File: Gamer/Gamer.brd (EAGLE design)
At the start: 168.9 x 63.5 mm, 44 parts, among them J1 HEADER-1X8, J2 HEADER-1X8, J3 HEADER-1X8, J4 HEADER-1X8, J5 HEADER-1X8, J6 HEADER-1X8, J7 HEADER-1X8, J8 HEADER-1X8, U1 MMA8653FCR1, U2 ATTINY48, U3 ULN2803AFWG, U4 ATTINY48, U5 ULN2803AFWG, U6 ATTINY48, U7 ULN2803AFWG, U8 ATTINY48, U9 ULN2803AFWG

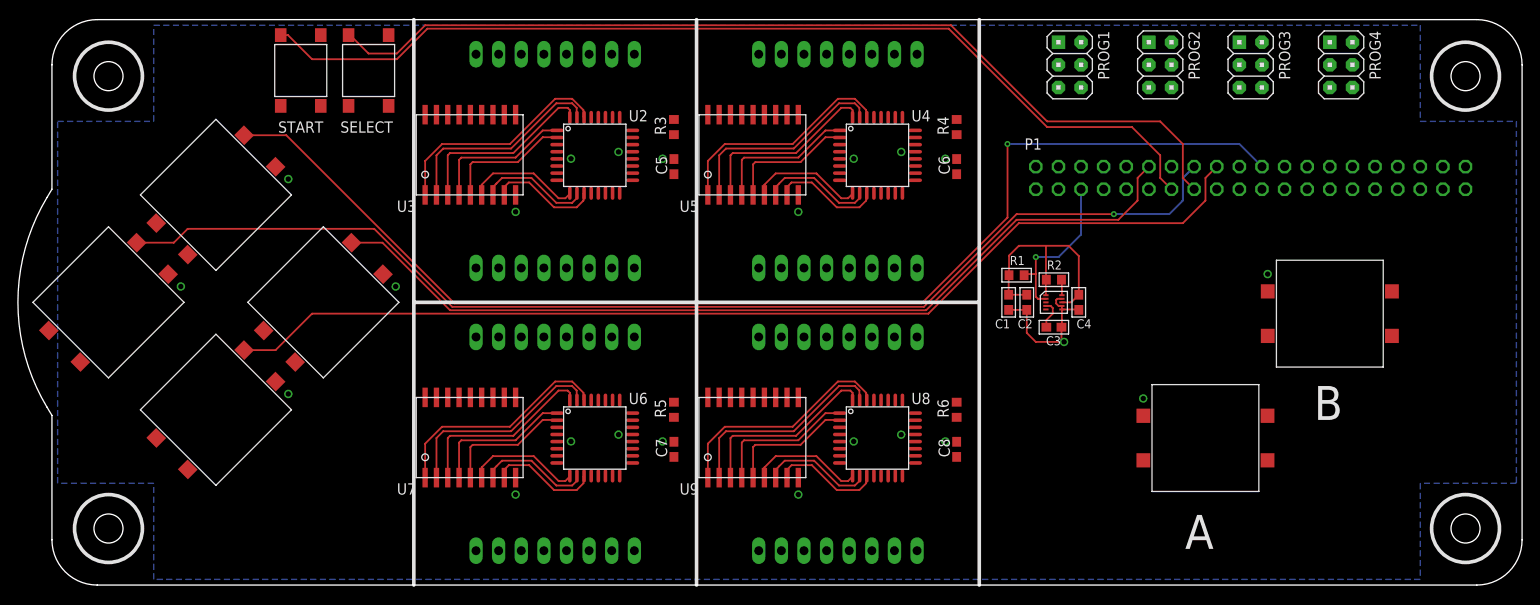
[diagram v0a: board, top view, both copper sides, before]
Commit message: gamer - auto route 100%
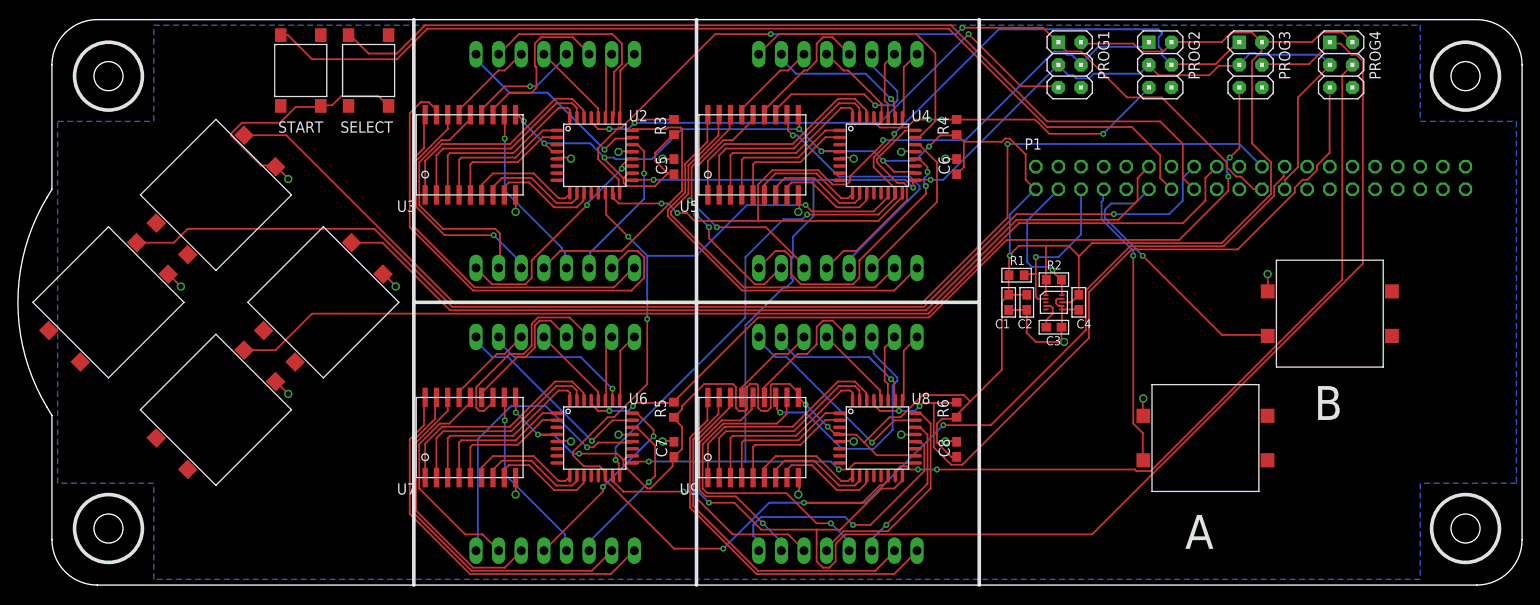
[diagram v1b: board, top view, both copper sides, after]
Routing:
- net 3V3: track 27.4 -> 328.0 mm, vias 0 -> 13
- net 8/CE0: track 0.00 -> 183.5 mm, vias 0 -> 6
- net 11/SCLK: track 0.00 -> 172.0 mm, vias 0 -> 5
- net MOSI3/MISO4: track 0.00 -> 154.7 mm, vias 0 -> 2
- net MOSI2/MISO3: track 0.00 -> 107.8 mm, vias 0 -> 3
- net M3_RESET: track 0.00 -> 94.8 mm, vias 0 -> 4
- net 9/MISO: track 0.00 -> 94.1 mm, vias 0 -> 2
- net MOSI1/MISO2: track 0.00 -> 93.4 mm, vias 0 -> 3
- net M4_RESET: track 0.00 -> 86.2 mm, vias 0 -> 2
- net 10/MISO: track 0.00 -> 84.7 mm, vias 0 -> 2
- net GND: track 17.2 -> 82.0 mm
- net M1_RESET: track 0.00 -> 64.8 mm, vias 0 -> 3
- net M1_COL1: track 0.00 -> 54.1 mm
- net M2_COL0: track 0.00 -> 45.8 mm
- net M3_COL0: track 0.00 -> 42.9 mm
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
